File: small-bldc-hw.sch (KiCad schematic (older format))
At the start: 48 parts, among them J1 More IO, J2 TEMP, J3 CONN_01X01, J4 CONN_01X01, J5 CONN_01X01, J6 CAN, J7 I2C, J8 CONN_01X01, J9 CONN_01X01, P1 CONN_02X01, P2 SWD, U1 STM32F042C6T6, Y1 16MHz

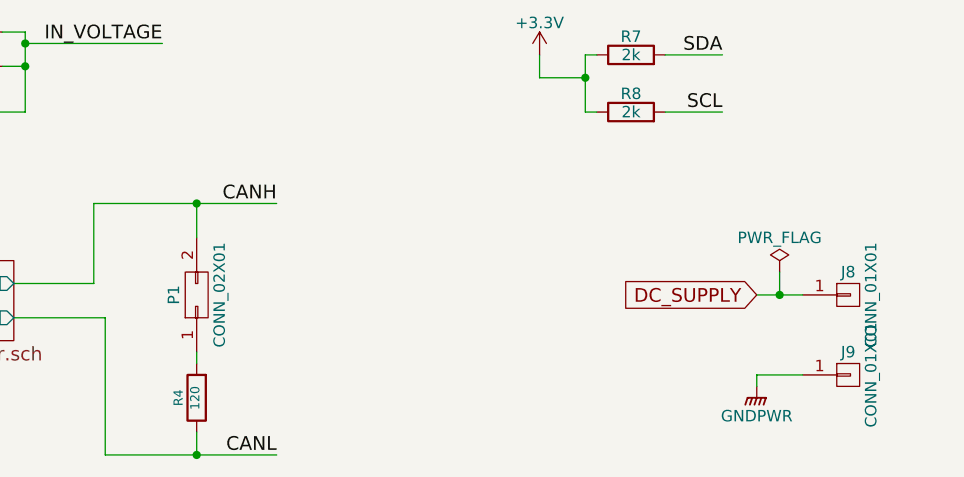
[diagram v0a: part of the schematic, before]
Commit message: stuff
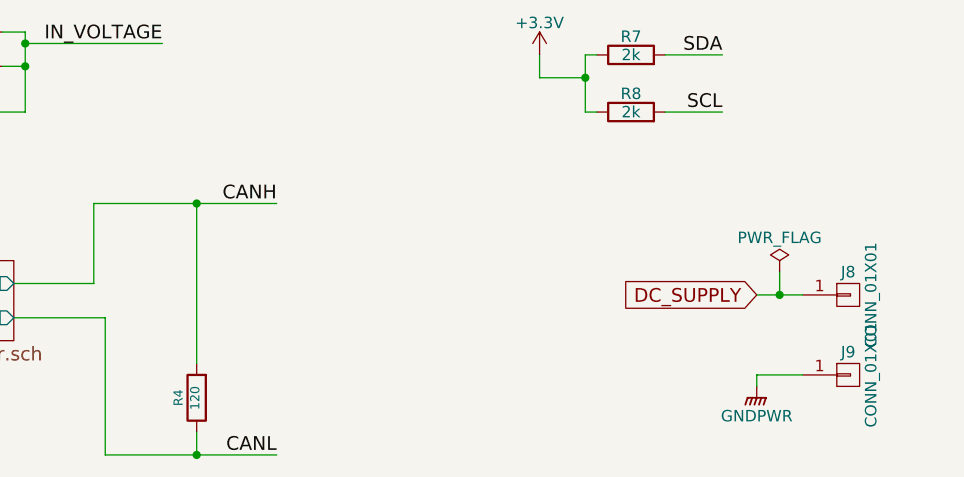
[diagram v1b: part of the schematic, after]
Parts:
- removed P1: CONN_02X01, Resistors_SMD:R_0402, symbol CONN_02X01
- J3, J4, J5: footprint Wire_Pads:SolderWirePad_single_SMD_5x10mm -> hlib:SolderWirePad_single_SMD_5x3.5mm
- J8, J9: footprint Wire_Pads:SolderWirePad_single_SMD_5x10mm -> hlib:SolderWirePad_single_SMD_5x3.5mm_holes
- JP1: footprint Pin_Headers:Pin_Header_Straight_1x02 -> Resistors_SMD:R_0603_HandSoldering
- Y1: footprint Crystals:Crystal_SMD_3225-4pin_3.2x2.5mm -> hlib:Crystal_SMD_3225-4pin_3.2x2.5mm
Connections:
- net CANH: now also R4.2
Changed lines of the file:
@@
-$EndComp
-$Comp
-L CONN_02X01 P1
-U 1 1 58D4CE36
-P 2750 6700
-F 0 "P1" H 2750 6800 50  0000 C CNN
-F 1 "CONN_02X01" H 2750 6600 50  0000 C CNN
-F 2 "Resistors_SMD:R_0402" H 2750 5500 50  0001 C CNN
-F 3 "" H 2750 5500 50  0000 C CNN
-	1    2750 6700
-	0    -1   -1   0
 $EndComp
 $Comp
@@
 F 0 "JP1" H 1700 2800 50  0000 C CNN
 F 1 "Boot Mode" H 1700 2700 50  0000 C CNN
-F 2 "Pin_Headers:Pin_Header_Straight_1x02" H 1700 1700 60  0001 C CNN
+F 2 "Resistors_SMD:R_0603_HandSoldering" H 1700 1700 60  0001 C CNN
 F 3 "" H 1700 1700 60  0000 C CNN
 	1    1700 2900
@@
 F 0 "J4" H 10450 4600 50  0000 C CNN
 F 1 "CONN_01X01" V 10550 4500 50  0001 C CNN
-F 2 "Wire_Pads:SolderWirePad_single_SMD_5x10mm" H 10450 4500 50  0001 C CNN
+F 2 "hlib:SolderWirePad_single_SMD_5x3.5mm" H 10450 4500 50  0001 C CNN
 F 3 "" H 10450 4500 50  0001 C CNN
 	1    10450 4500
@@
 F 0 "J3" H 10450 4100 50  0000 C CNN
 F 1 "CONN_01X01" V 10550 4000 50  0001 C CNN
-F 2 "Wire_Pads:SolderWirePad_single_SMD_5x10mm" H 10450 4000 50  0001 C CNN
+F 2 "hlib:SolderWirePad_single_SMD_5x3.5mm" H 10450 4000 50  0001 C CNN
 F 3 "" H 10450 4000 50  0001 C CNN
 	1    10450 4000
@@
 F 0 "J5" H 10450 5100 50  0000 C CNN
 F 1 "CONN_01X01" V 10550 5000 50  0001 C CNN
-F 2 "Wire_Pads:SolderWirePad_single_SMD_5x10mm" H 10450 5000 50  0001 C CNN
+F 2 "hlib:SolderWirePad_single_SMD_5x3.5mm" H 10450 5000 50  0001 C CNN
 F 3 "" H 10450 5000 50  0001 C CNN
 	1    10450 5000
@@
 $EndComp
 Wire Wire Line
-	2750 7000 2750 6950
-Wire Wire Line
 	1950 6650 2300 6650
 Wire Wire Line
@@
 	2350 7400 3100 7400
 Wire Wire Line
-	2750 6450 2750 6300
+	2750 7000 2750 6300
 Connection ~ 2750 6300
 Wire Wire Line
@@
 F 0 "J8" H 5600 6800 50  0000 C CNN
 F 1 "CONN_01X01" V 5700 6700 50  0000 C CNN
-F 2 "Wire_Pads:SolderWirePad_single_SMD_5x10mm" H 5600 6700 50  0001 C CNN
+F 2 "hlib:SolderWirePad_single_SMD_5x3.5mm_holes" H 5600 6700 50  0001 C CNN
 F 3 "" H 5600 6700 50  0001 C CNN
 	1    5600 6700
@@
 $EndComp
 Wire Wire Line
-	5400 6700 5200 6700
+	5200 6700 5400 6700
 $Comp
 L CONN_01X01 J9
@@
 F 0 "J9" H 5600 7150 50  0000 C CNN
 F 1 "CONN_01X01" V 5700 7050 50  0000 C CNN
-F 2 "Wire_Pads:SolderWirePad_single_SMD_5x10mm" H 5600 7050 50  0001 C CNN
+F 2 "hlib:SolderWirePad_single_SMD_5x3.5mm_holes" H 5600 7050 50  0001 C CNN
 F 3 "" H 5600 7050 50  0001 C CNN
 	1    5600 7050
@@
 F 0 "Y1" H 1025 3250 50  0000 L CNN
 F 1 "16MHz" H 1025 3175 50  0000 L CNN
-F 2 "Crystals:Crystal_SMD_3225-4pin_3.2x2.5mm" H 900 3050 50  0001 C CNN
+F 2 "hlib:Crystal_SMD_3225-4pin_3.2x2.5mm" H 900 3050 50  0001 C CNN
 F 3 "" H 900 3050 50  0001 C CNN
 F 4 "FA-238 16.0000MB-K3" H 900 3050 60  0001 C CNN "MPN"

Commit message: BOM stuff
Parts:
- J3, J4, J5: footprint hlib:SolderWirePad_single_SMD_5x3.5mm -> hlib:SolderWirePad_single_SMD_5x3.5mm_holes
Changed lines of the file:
@@
 F 0 "J4" H 10450 4600 50  0000 C CNN
 F 1 "CONN_01X01" V 10550 4500 50  0001 C CNN
-F 2 "hlib:SolderWirePad_single_SMD_5x3.5mm" H 10450 4500 50  0001 C CNN
+F 2 "hlib:SolderWirePad_single_SMD_5x3.5mm_holes" H 10450 4500 50  0001 C CNN
 F 3 "" H 10450 4500 50  0001 C CNN
 	1    10450 4500
@@
 F 0 "J3" H 10450 4100 50  0000 C CNN
 F 1 "CONN_01X01" V 10550 4000 50  0001 C CNN
-F 2 "hlib:SolderWirePad_single_SMD_5x3.5mm" H 10450 4000 50  0001 C CNN
+F 2 "hlib:SolderWirePad_single_SMD_5x3.5mm_holes" H 10450 4000 50  0001 C CNN
 F 3 "" H 10450 4000 50  0001 C CNN
 	1    10450 4000
@@
 F 0 "J5" H 10450 5100 50  0000 C CNN
 F 1 "CONN_01X01" V 10550 5000 50  0001 C CNN
-F 2 "hlib:SolderWirePad_single_SMD_5x3.5mm" H 10450 5000 50  0001 C CNN
+F 2 "hlib:SolderWirePad_single_SMD_5x3.5mm_holes" H 10450 5000 50  0001 C CNN
 F 3 "" H 10450 5000 50  0001 C CNN
 	1    10450 5000
